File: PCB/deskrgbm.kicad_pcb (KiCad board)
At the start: 2 copper layers, 83 x 103 mm, 132 parts, among them SW1 RotaryEncoder_Switch_MP, U1 XIAO-RP2040-DIP

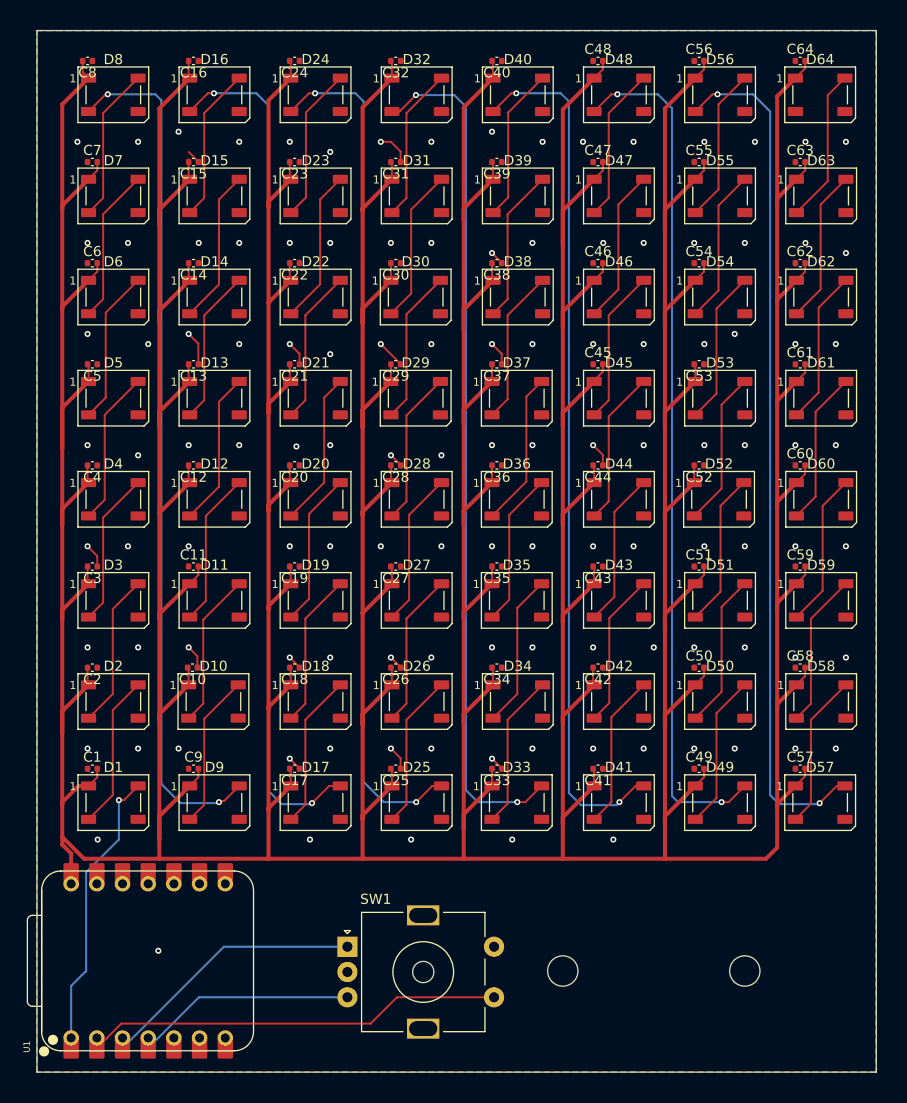
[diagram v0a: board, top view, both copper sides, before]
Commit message: Journal + CAD
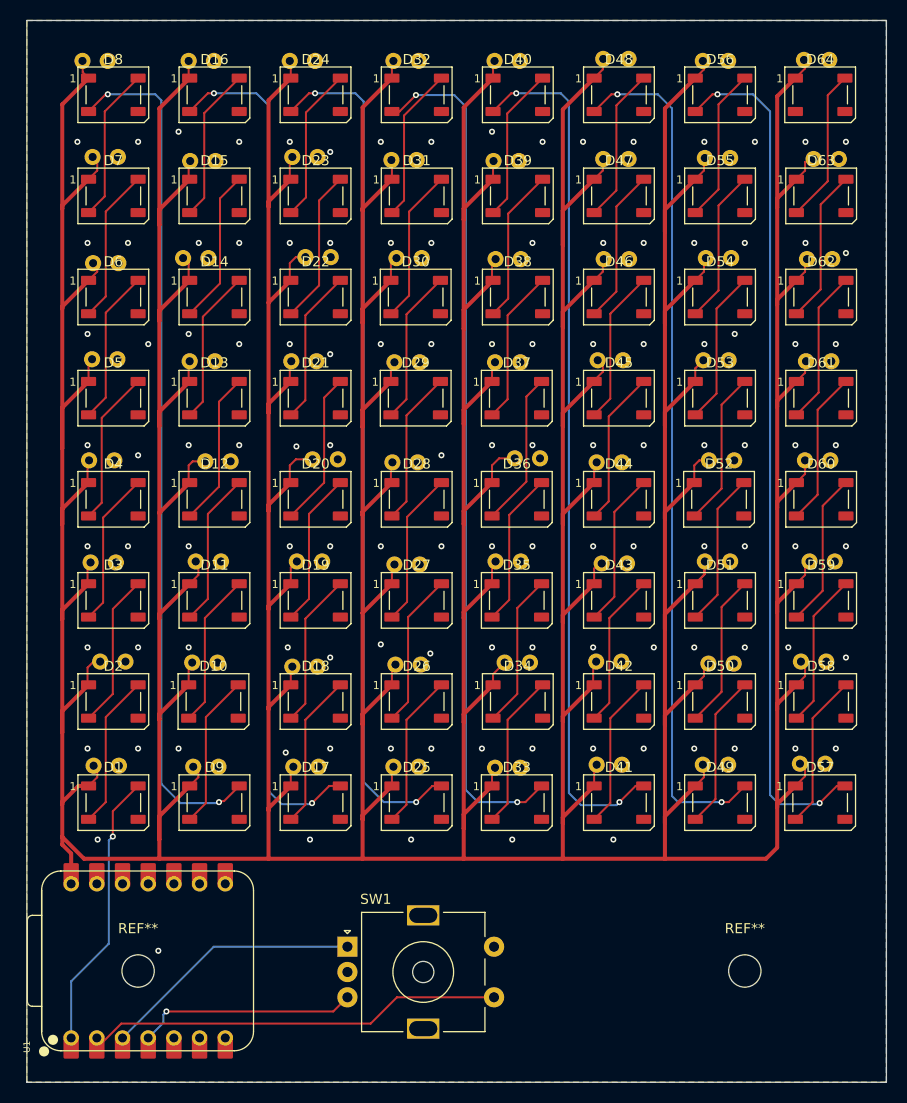
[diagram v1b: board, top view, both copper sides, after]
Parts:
- removed the REF** at (150.0, 110.0)
- removed the REF** at (132.0, 110.0)
- added REF**: MountingHole_3.2mm_M3, MountingHole:MountingHole_3.2mm_M3, F.Cu at (150.0, 110.0)
- added REF**: MountingHole_3.2mm_M3, MountingHole:MountingHole_3.2mm_M3, F.Cu at (90.0, 110.0)
- C1, C10, C11, C12, C13, C14, C15, C16, C17, C18, C19, C2, C20, C21, C22, C23, C24, C25, C26, C27, C28, C29, C3, C30, C31, C32, C33, C34, C35, C36, C37, C38, C39, C4, C40, C41, C42, C43, C44, C45, C46, C47, C48, C49, C5, C50, C51, C52, C53, C54, C55, C56, C57, C58, C59, C6, C60, C61, C62, C63, C64, C7, C8, C9: footprint Capacitor_SMD:C_0402_1005Metric -> Capacitor_THT:C_Disc_D3.0mm_W1.6mm_P2.50mm; moved to B.Cu
- moved C36 4.33 mm to (129.8, 59.3)
- moved C20 4.31 mm to (109.8, 59.4)
- moved C63 3.83 mm to (159.3, 29.7), turned to 180 degrees
- moved C12 3.69 mm to (99.2, 59.6)
- moved C22 3.62 mm to (109.0, 39.4)
- moved C52 3.51 mm to (148.9, 59.5)
- moved C59 3.46 mm to (158.9, 69.5), turned to 180 degrees
- moved C50 3.44 mm to (148.9, 79.6), turned to 180 degrees
- moved C2 3.32 mm to (88.8, 79.4)
- moved C34 3.31 mm to (128.8, 79.5)
- moved C54 3.21 mm to (148.7, 39.5), turned to 180 degrees
- moved C62 3.20 mm to (158.7, 39.6), turned to 180 degrees
- moved C51 3.11 mm to (148.6, 69.5), turned to 180 degrees
- moved C46 3.10 mm to (138.6, 39.6), turned to 180 degrees
- moved C55 3.10 mm to (148.6, 29.6), turned to 180 degrees
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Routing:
- net GND: track 33.7 -> 0.00 mm, vias 115 -> 113
- net 5V: track 1084.9 -> 1103.3 mm
- net Net-(D1-DIN): track 30.0 -> 27.7 mm
- net ENC_B: vias 0 -> 1
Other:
- board size 83 x 103 mm -> 85 x 105 mm
